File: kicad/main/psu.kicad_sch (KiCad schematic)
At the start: 2 parts, among them J1 ATX-24, J2 Conn_01x02_Pin

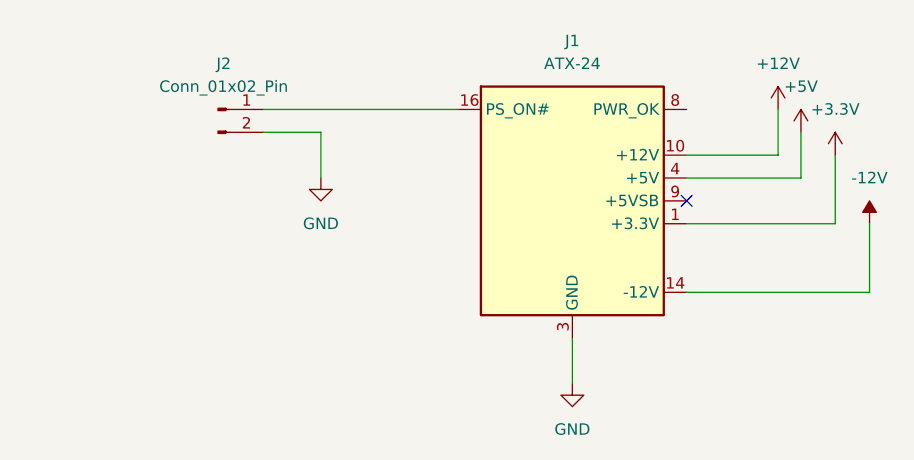
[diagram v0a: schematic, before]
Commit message: gonna see if i can switch back to linux
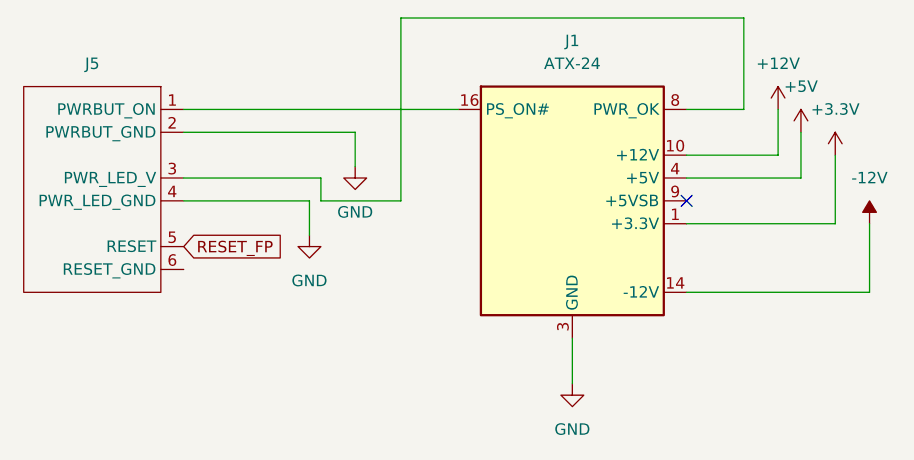
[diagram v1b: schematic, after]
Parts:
- removed J2: Conn_01x02_Pin, Connector_JST:JST_EH_B2B-EH-A_1x02_P2.50mm_Vertical, symbol Connector:Conn_01x02_Pin
- added J5: (no value), Connector_PinHeader_2.54mm:PinHeader_2x03_P2.54mm_Vertical, symbol az030:FP_HEADER
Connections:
- net GND: now also J5.2 (PWRBUT_GND), J5.4 (PWR_LED_GND)
- net at J1.16 (PS_ON#): now also J5.1 (PWRBUT_ON)
- net at J1.8 (PWR_OK): now also J5.3 (PWR_LED_V)
- new net RESET_FP: J5.5 (RESET)
